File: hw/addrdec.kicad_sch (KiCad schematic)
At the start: 5 parts, among them U10 74AS138, U11 74ACT00P, U5 74AHCT02, U8 74AS04N, U9 74AS27

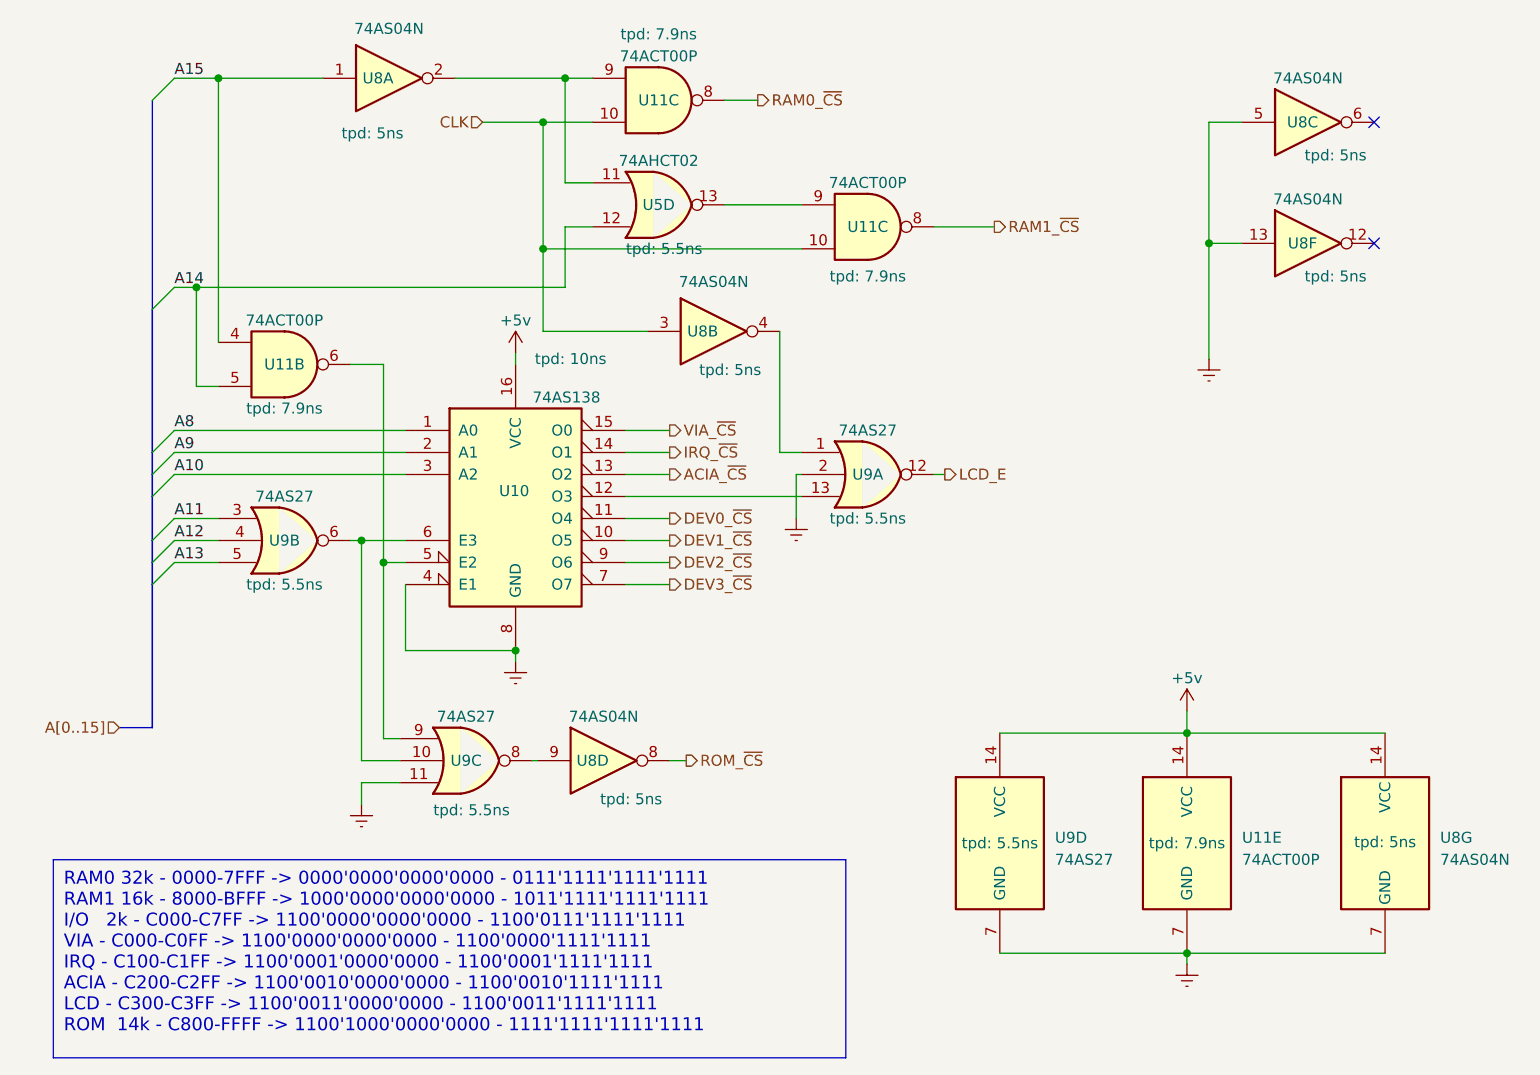
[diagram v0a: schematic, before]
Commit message: add hw design for veraduino
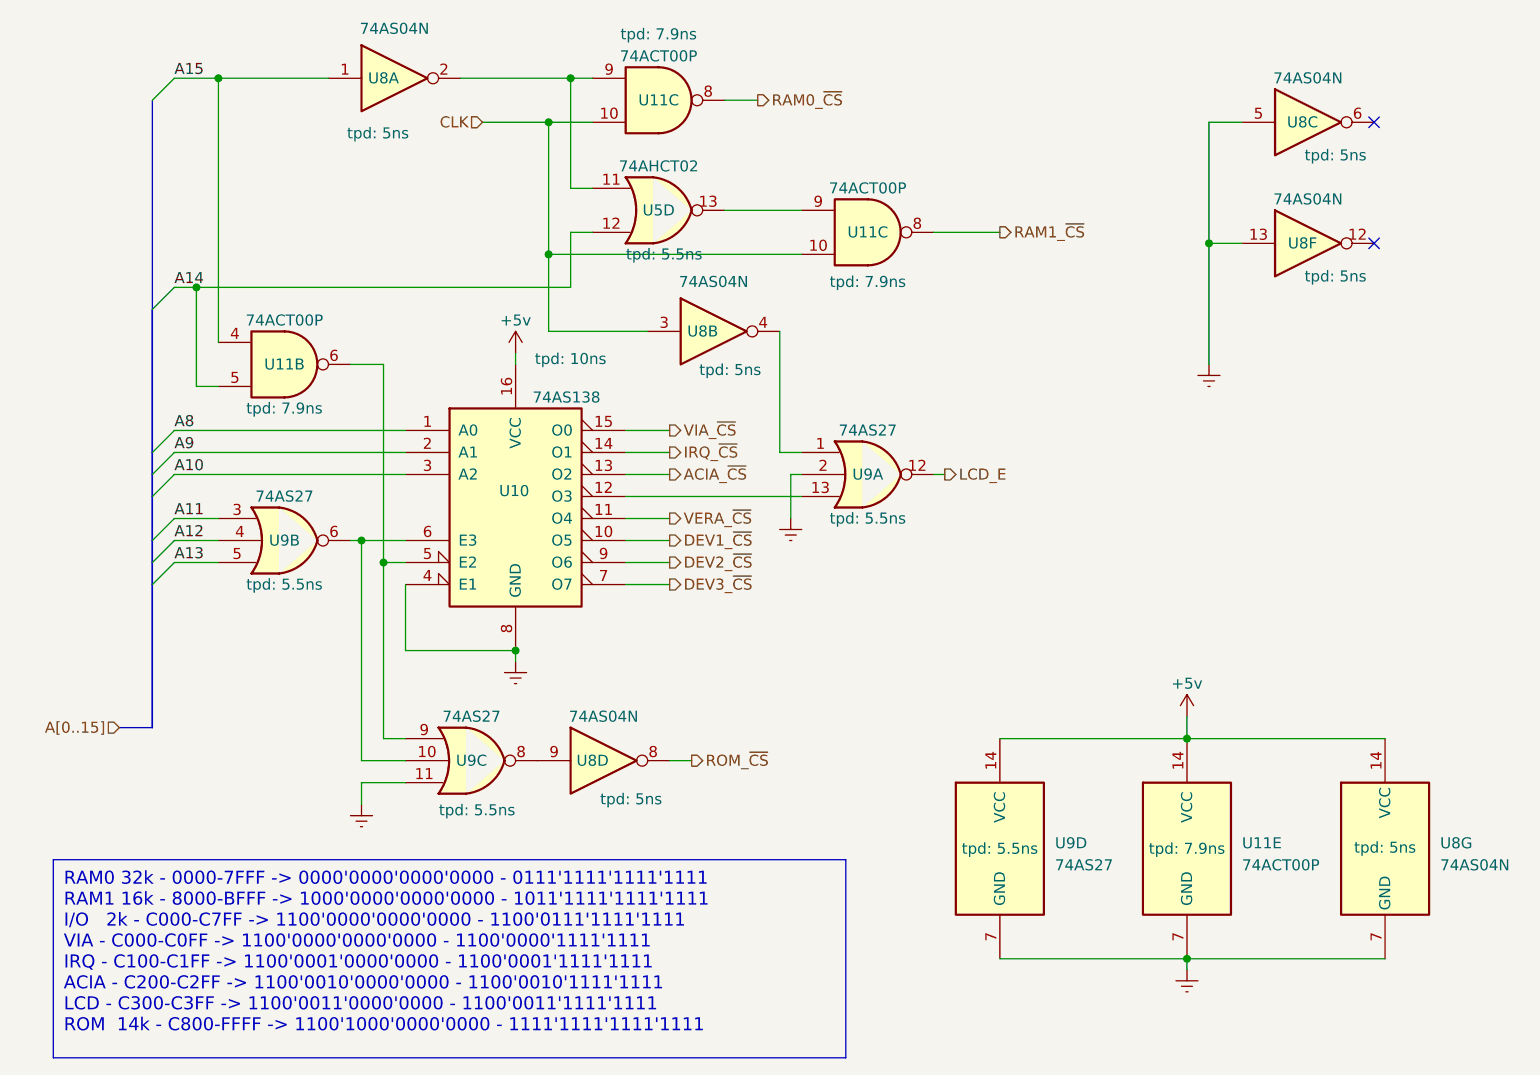
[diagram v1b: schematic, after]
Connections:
- net DEV0_~{CS} renamed VERA_~{CS}
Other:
- moved on the sheet: U11C, U11E, U5D, U8A, U8G, U9C, U9D
